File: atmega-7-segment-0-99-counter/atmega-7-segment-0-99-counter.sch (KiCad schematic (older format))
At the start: 2 parts

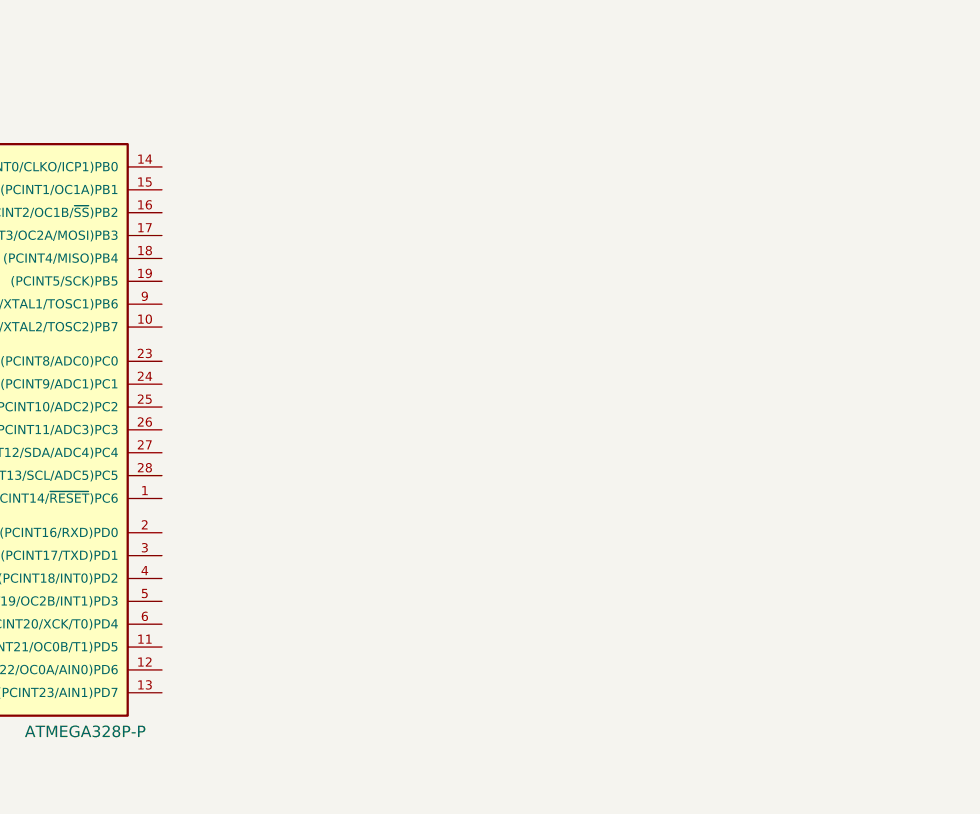
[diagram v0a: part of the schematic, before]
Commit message: Updated schematics
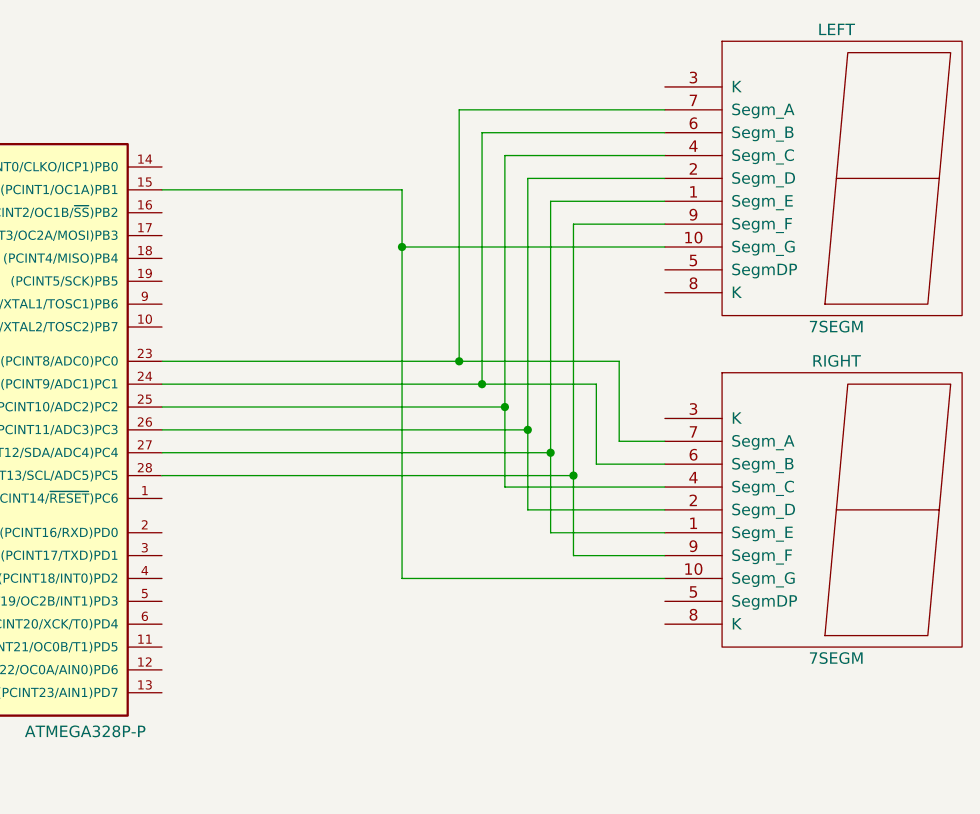
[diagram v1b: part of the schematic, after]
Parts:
- added LEFT, RIGHT: 7SEGM, symbol 7SEGM
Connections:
- net at IC?.15 ((PCINT1/OC1A)PB1): now also LEFT.10 (Segm_G), RIGHT.10 (Segm_G)
- net at IC?.23 ((PCINT8/ADC0)PC0): now also LEFT.7 (Segm_A), RIGHT.7 (Segm_A)
- net at IC?.24 ((PCINT9/ADC1)PC1): now also LEFT.6 (Segm_B), RIGHT.6 (Segm_B)
- net at IC?.25 ((PCINT10/ADC2)PC2): now also LEFT.4 (Segm_C), RIGHT.4 (Segm_C)
- net at IC?.26 ((PCINT11/ADC3)PC3): now also LEFT.2 (Segm_D), RIGHT.2 (Segm_D)
- net at IC?.27 ((PCINT12/SDA/ADC4)PC4): now also LEFT.1 (Segm_E), RIGHT.1 (Segm_E)
- net at IC?.28 ((PCINT13/SCL/ADC5)PC5): now also LEFT.9 (Segm_F), RIGHT.9 (Segm_F)
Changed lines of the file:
@@
 	4950 4900 4700 4900
 Connection ~ 4700 4900
+$Comp
+L 7SEGM LEFT
+U 1 1 57D020AC
+P 9800 2650
+F 0 "LEFT" H 9800 3300 50  0000 C CNN
+F 1 "7SEGM" H 9800 2000 50  0000 C CNN
+F 2 "" H 9800 2650 50  0000 C CNN
+F 3 "" H 9800 2650 50  0000 C CNN
+	1    9800 2650
+	1    0    0    -1
+$EndComp
+$Comp
+L 7SEGM RIGHT
+U 1 1 57D0216C
+P 9800 4100
+F 0 "RIGHT" H 9800 4750 50  0000 C CNN
+F 1 "7SEGM" H 9800 3450 50  0000 C CNN
+F 2 "" H 9800 4100 50  0000 C CNN
+F 3 "" H 9800 4100 50  0000 C CNN
+	1    9800 4100
+	1    0    0    -1
+$EndComp
+Wire Wire Line
+	6850 3450 8850 3450
+Wire Wire Line
+	8150 3450 8150 2350
+Wire Wire Line
+	8150 2350 9050 2350
+Wire Wire Line
+	6850 3550 8750 3550
+Wire Wire Line
+	8250 3550 8250 2450
+Wire Wire Line
+	8250 2450 9050 2450
+Wire Wire Line
+	6850 3650 8350 3650
+Wire Wire Line
+	8350 2550 9050 2550
+Wire Wire Line
+	6850 3750 8450 3750
+Wire Wire Line
+	8450 2650 8450 4100
+Wire Wire Line
+	8450 2650 9050 2650
+Wire Wire Line
+	6850 3850 8550 3850
+Wire Wire Line
+	8550 2750 8550 4200
+Wire Wire Line
+	8550 2750 9050 2750
+Wire Wire Line
+	6850 3950 8650 3950
+Wire Wire Line
+	8650 2850 8650 4300
+Wire Wire Line
+	8650 2850 9050 2850
+Wire Wire Line
+	8650 4300 9050 4300
+Connection ~ 8650 3950
+Wire Wire Line
+	8550 4200 9050 4200
+Connection ~ 8550 3850
+Wire Wire Line
+	8450 4100 9050 4100
+Connection ~ 8450 3750
+Wire Wire Line
+	8350 2550 8350 4000
+Wire Wire Line
+	8350 4000 9050 4000
+Connection ~ 8350 3650
+Wire Wire Line
+	8750 3550 8750 3900
+Wire Wire Line
+	8750 3900 9050 3900
+Connection ~ 8250 3550
+Wire Wire Line
+	8850 3450 8850 3800
+Wire Wire Line
+	8850 3800 9050 3800
+Connection ~ 8150 3450
+Wire Wire Line
+	7900 4400 9050 4400
+Wire Wire Line
+	6850 2700 7900 2700
+Wire Wire Line
+	7900 2700 7900 4400
+Wire Wire Line
+	9050 2950 7900 2950
+Connection ~ 7900 2950
 $EndSCHEMATC

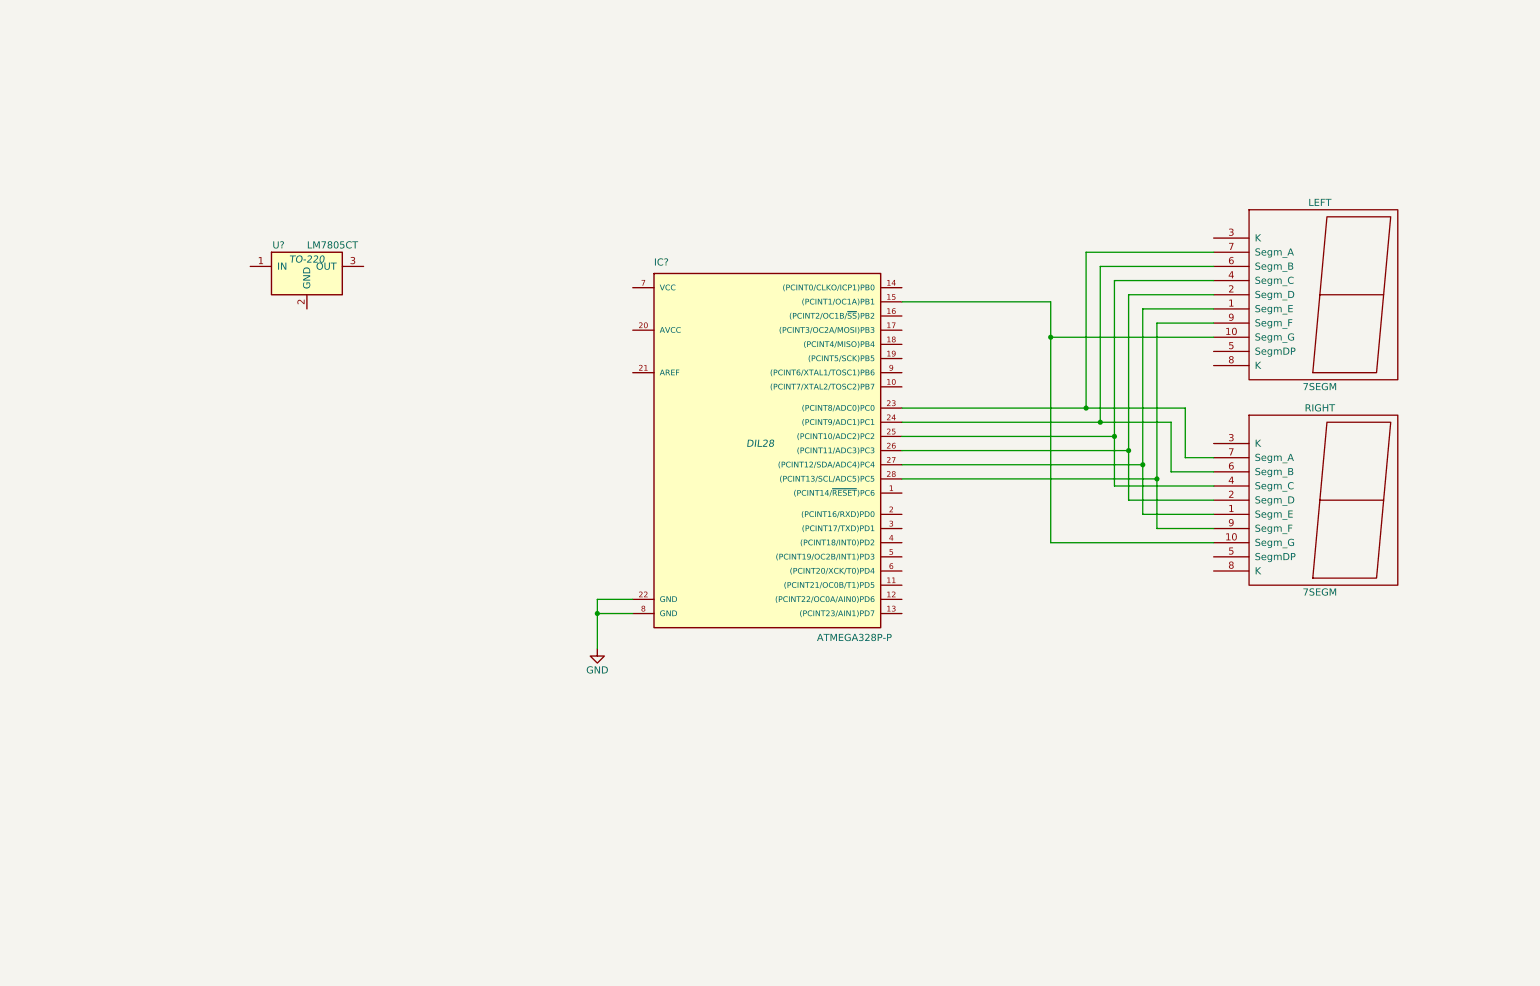
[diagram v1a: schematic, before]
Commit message: Progress on schematics
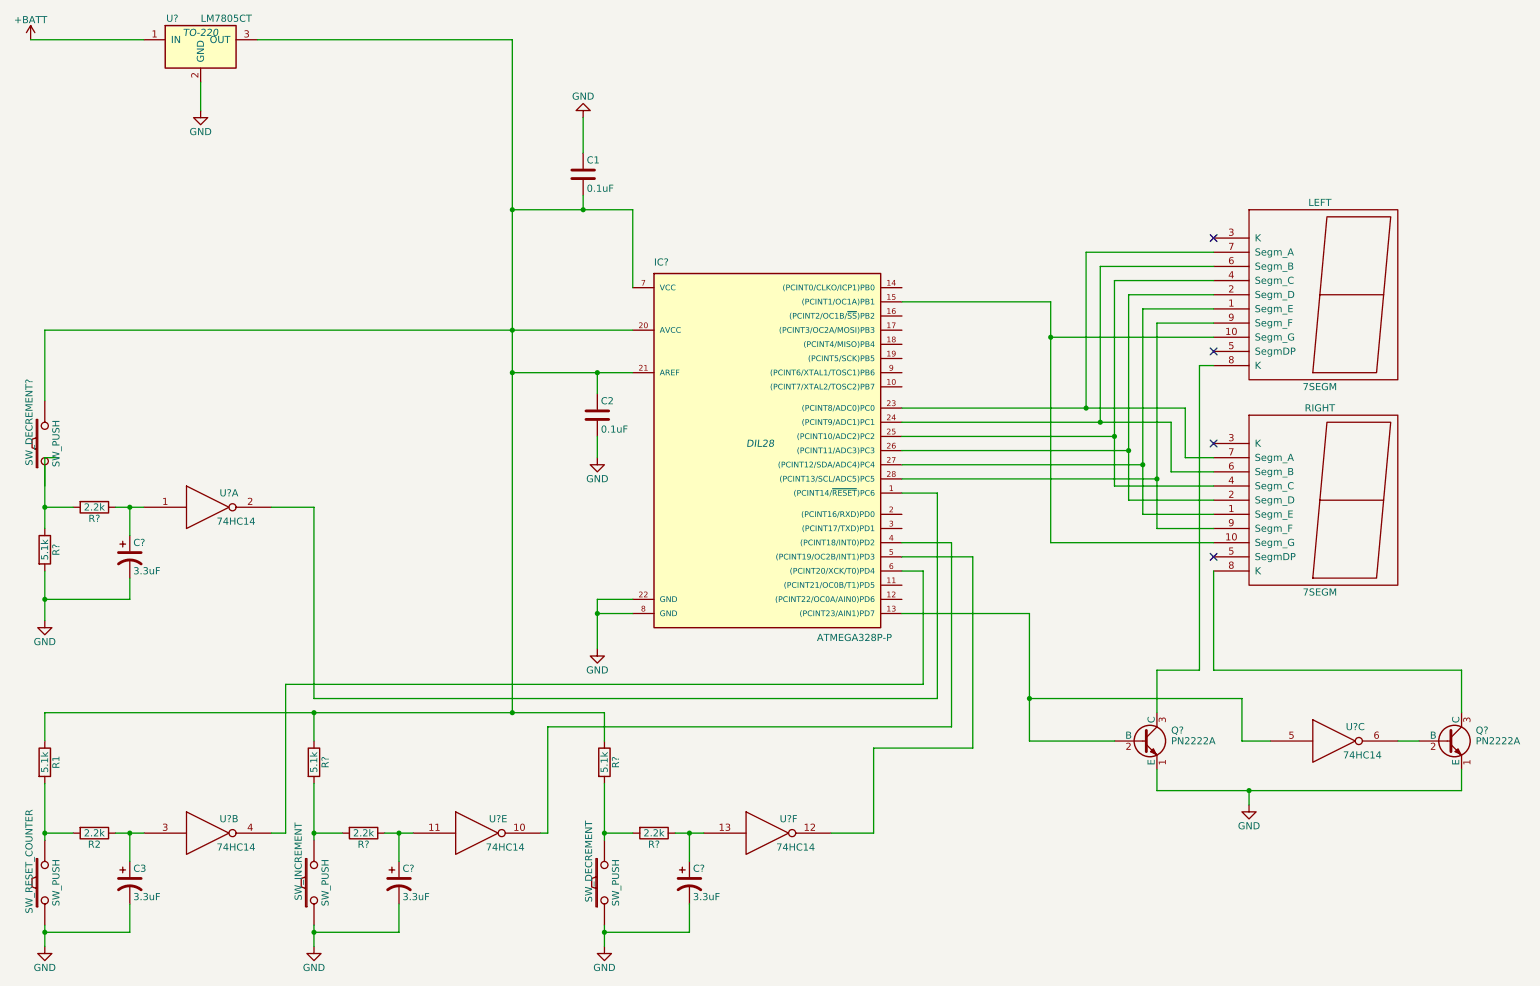
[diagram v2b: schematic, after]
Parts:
- added C1, C2: 0.1uF, symbol C
- added C3, C? (x3): 3.3uF, symbol CP1
- added Q? (x2): PN2222A, symbol PN2222A
- added R1, R? (x3): 5.1k, symbol R
- added R2, R? (x3): 2.2k, symbol R
- added SW_DECREMENT, SW_DECREMENT?, SW_INCREMENT, SW_RESET_COUNTER: SW_PUSH, symbol SW_PUSH
- added U? (x5): 74HC14, symbol 74HC14
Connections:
- net GND: now also U?.2 (GND), C1.1, C2.2, C3.2, C?.2, C?.2, C?.2, Q?.1 (E), Q?.1 (E), R?.2, SW_DECREMENT.1, SW_INCREMENT.1, SW_RESET_COUNTER.1, U?.7 (GND), U?.7 (GND), U?.7 (GND), U?.7 (GND), U?.7 (GND)
- net +BATT: now reaches U?.1 (IN)
- net at U?.3 (OUT): now also IC?.20 (AVCC), IC?.21 (AREF), IC?.7 (VCC), C1.2, C2.1, R1.1, R?.1, R?.1, SW_DECREMENT?.2
- net at IC?.1 ((PCINT14/~RESET~)PC6): now also U?.2
- net at IC?.13 ((PCINT23/AIN1)PD7): now also Q?.2 (B), U?.5
- net at IC?.4 ((PCINT18/INT0)PD2): now also U?.10
- net at IC?.5 ((PCINT19/OC2B/INT1)PD3): now also U?.12
- net at IC?.6 ((PCINT20/XCK/T0)PD4): now also U?.4
- net at LEFT.8 (K): now also Q?.3 (C)
- net at RIGHT.8 (K): now also Q?.3 (C)
- new net: R1.2, R2.2, SW_RESET_COUNTER.2
- new net: C3.1, R2.1, U?.3
- new net: Q?.2 (B), U?.6
- new net: R?.2, R?.2, SW_INCREMENT.2
- new net: C?.1, R?.1, U?.11
- new net: R?.2, R?.2, SW_DECREMENT.2
- new net: C?.1, R?.1, U?.13
- new net: R?.1, R?.2
- new net: C?.1, R?.1, U?.1
- new net VCC: U?.14 (VCC), U?.14 (VCC), U?.14 (VCC), U?.14 (VCC), U?.14 (VCC)
- no-connect marks 0 -> 4
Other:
- moved on the sheet: U?
